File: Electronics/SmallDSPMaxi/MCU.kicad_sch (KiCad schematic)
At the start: 47 parts, among them J21 Header, J22 Header, J23 Header, J24 Header, Q2 2N7002, Q3 2N7002, Q4 2N7002, SW3 TS-1187A-B-A-B, U14 STM32F030C8Tx, Y2 8MHz

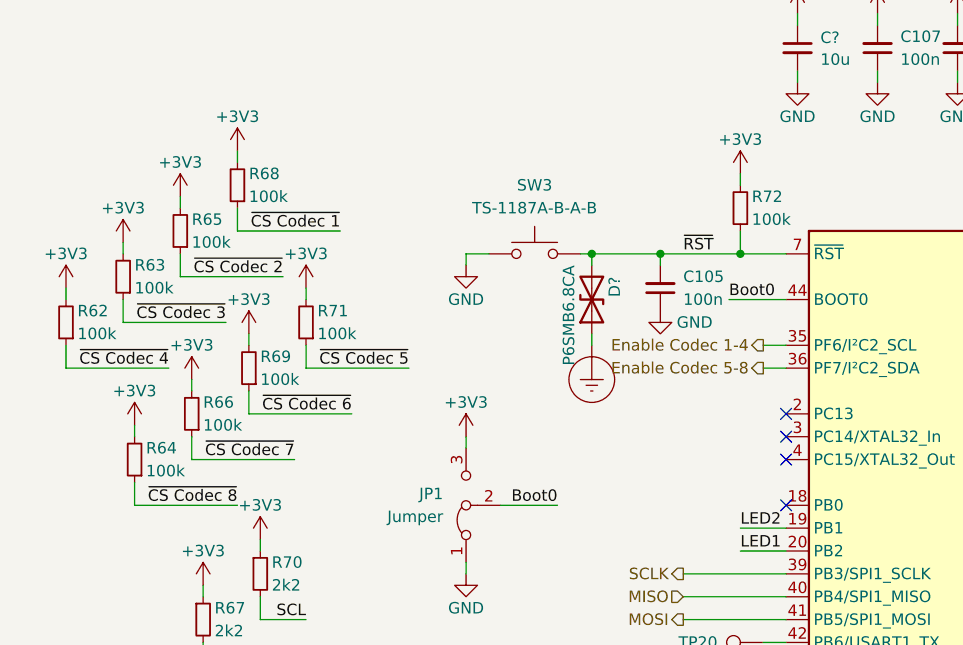
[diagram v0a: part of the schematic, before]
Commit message: Fixes minor issues
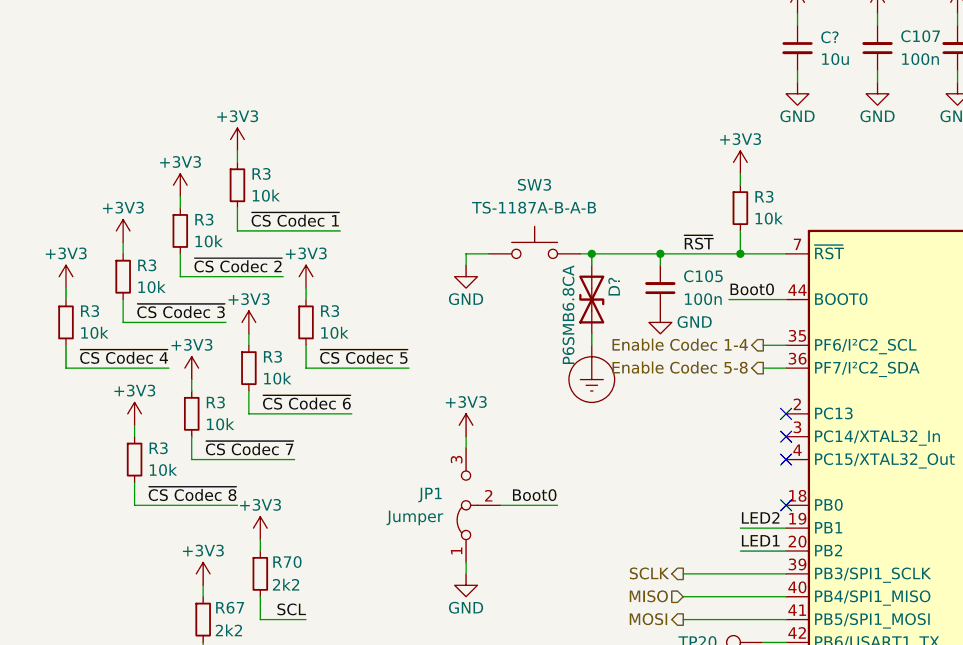
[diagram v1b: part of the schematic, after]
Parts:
- removed R62, R63, R64, R65, R66, R68, R69, R71, R72: 100k, Resistor_SMD:R_0402_1005Metric, symbol Device:R_Small
- added R3 (x9): 10k, Resistor_SMD:R_0402_1005Metric, symbol Device:R_Small
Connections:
- net +3V3: now also R3.1, R3.1, R3.1, R3.1, R3.1, R3.1, R3.1, R3.1, R3.1
- net ~{CS Codec 1}: now also R3.2
- net ~{CS Codec 2}: now also R3.2
- net ~{CS Codec 3}: now also R3.2
- net ~{CS Codec 4}: now also R3.2
- net ~{CS Codec 5}: now also R3.2
- net ~{CS Codec 6}: now also R3.2
- net ~{CS Codec 7}: now also R3.2
- net ~{CS Codec 8}: now also R3.2
- net ~{RST}: now also R3.2
